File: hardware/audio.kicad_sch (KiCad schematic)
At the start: 3 parts, among them J5 AudioJack4

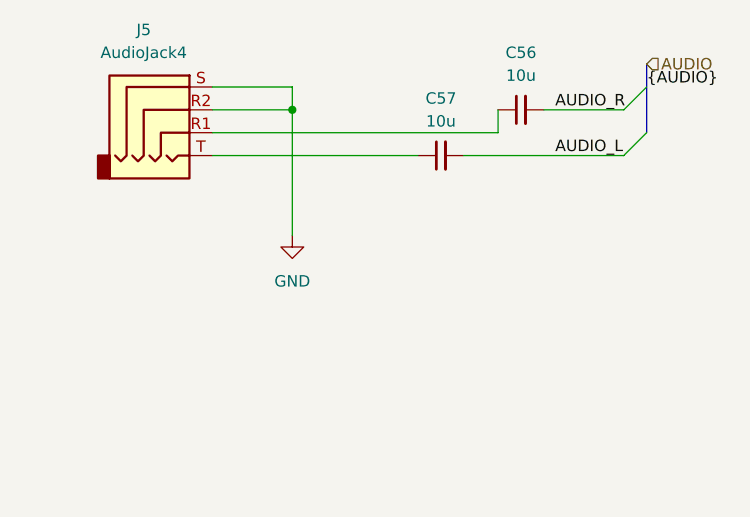
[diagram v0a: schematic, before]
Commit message: final touches
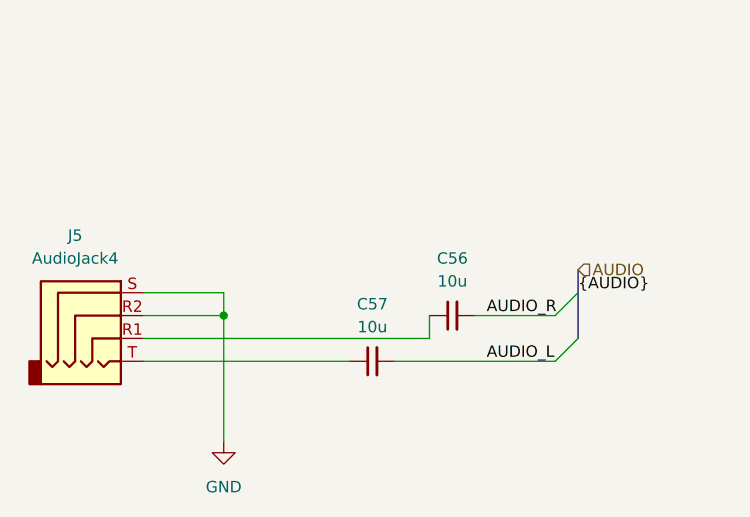
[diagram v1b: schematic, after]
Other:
- moved on the sheet: C56, C57, J5
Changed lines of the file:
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@@
 	(paper "A4")
 	(junction
-		(at 144.78 71.12)
+		(at 137.16 93.98)
 		(diameter 0)
 		(color 0 0 0 0)
 	)
 	(bus_entry
-		(at 184.15 73.66)
+		(at 176.53 96.52)
 		(size -2.54 2.54)
 		(stroke
@@
 	)
 	(bus_entry
-		(at 184.15 68.58)
+		(at 176.53 91.44)
 		(size -2.54 2.54)
 		(stroke
@@
 	(wire
 		(pts
-			(xy 135.89 71.12) (xy 144.78 71.12)
-		)
-		(stroke
-			(width 0)
-			(type default)
-		)
-	)
-	(wire
-		(pts
-			(xy 163.83 76.2) (xy 181.61 76.2)
-		)
-		(stroke
-			(width 0)
-			(type default)
-		)
-	)
-	(wire
-		(pts
-			(xy 144.78 85.09) (xy 144.78 71.12)
-		)
-		(stroke
-			(width 0)
-			(type default)
-		)
-	)
-	(wire
-		(pts
-			(xy 135.89 76.2) (xy 158.75 76.2)
+			(xy 128.27 93.98) (xy 137.16 93.98)
+		)
+		(stroke
+			(width 0)
+			(type default)
+		)
+	)
+	(wire
+		(pts
+			(xy 156.21 99.06) (xy 173.99 99.06)
+		)
+		(stroke
+			(width 0)
+			(type default)
+		)
+	)
+	(wire
+		(pts
+			(xy 137.16 107.95) (xy 137.16 93.98)
+		)
+		(stroke
+			(width 0)
+			(type default)
+		)
+	)
+	(wire
+		(pts
+			(xy 128.27 99.06) (xy 151.13 99.06)
 		)
 		(stroke
@@
 	(bus
 		(pts
-			(xy 184.15 66.04) (xy 184.15 73.66)
-		)
-		(stroke
-			(width 0)
-			(type default)
-		)
-	)
-	(wire
-		(pts
-			(xy 135.89 73.66) (xy 167.64 73.66)
-		)
-		(stroke
-			(width 0)
-			(type default)
-		)
-	)
-	(wire
-		(pts
-			(xy 135.89 68.58) (xy 144.78 68.58)
-		)
-		(stroke
-			(width 0)
-			(type default)
-		)
-	)
-	(wire
-		(pts
-			(xy 167.64 73.66) (xy 167.64 71.12)
-		)
-		(stroke
-			(width 0)
-			(type default)
-		)
-	)
-	(wire
-		(pts
-			(xy 172.72 71.12) (xy 181.61 71.12)
-		)
-		(stroke
-			(width 0)
-			(type default)
-		)
-	)
-	(wire
-		(pts
-			(xy 144.78 71.12) (xy 144.78 68.58)
+			(xy 176.53 88.9) (xy 176.53 96.52)
+		)
+		(stroke
+			(width 0)
+			(type default)
+		)
+	)
+	(wire
+		(pts
+			(xy 128.27 96.52) (xy 160.02 96.52)
+		)
+		(stroke
+			(width 0)
+			(type default)
+		)
+	)
+	(wire
+		(pts
+			(xy 128.27 91.44) (xy 137.16 91.44)
+		)
+		(stroke
+			(width 0)
+			(type default)
+		)
+	)
+	(wire
+		(pts
+			(xy 160.02 96.52) (xy 160.02 93.98)
+		)
+		(stroke
+			(width 0)
+			(type default)
+		)
+	)
+	(wire
+		(pts
+			(xy 165.1 93.98) (xy 173.99 93.98)
+		)
+		(stroke
+			(width 0)
+			(type default)
+		)
+	)
+	(wire
+		(pts
+			(xy 137.16 93.98) (xy 137.16 91.44)
 		)
 		(stroke
@@
 	)
 	(label "AUDIO_L"
-		(at 173.99 76.2 0)
+		(at 166.37 99.06 0)
 		(effects
 			(font
@@
 	)
 	(label "{AUDIO}"
-		(at 184.15 68.58 0)
+		(at 176.53 91.44 0)
 		(effects
 			(font
@@
 	)
 	(label "AUDIO_R"
-		(at 173.99 71.12 0)
+		(at 166.37 93.98 0)
 		(effects
 			(font
@@
 	(hierarchical_label "AUDIO"
 		(shape input)
-		(at 184.15 66.04 0)
+		(at 176.53 88.9 0)
 		(effects
 			(font
@@
 	(symbol
 		(lib_id "power:GND")
-		(at 144.78 85.09 0)
+		(at 137.16 107.95 0)
 		(unit 1)
 		(body_style 1)
@@
 		(fields_autoplaced yes)
 		(property "Reference" "#PWR055"
-			(at 144.78 91.44 0)
+			(at 137.16 114.3 0)
 			(hide yes)
 			(show_name no)
@@
 		)
 		(property "Value" "GND"
-			(at 144.78 90.17 0)
+			(at 137.16 113.03 0)
 			(show_name no)
 			(do_not_autoplace no)
@@
 		)
 		(property "Footprint" ""
-			(at 144.78 85.09 0)
+			(at 137.16 107.95 0)
 			(hide yes)
 			(show_name no)
@@
 		)
 		(property "Datasheet" ""
-			(at 144.78 85.09 0)
+			(at 137.16 107.95 0)
 			(hide yes)
 			(show_name no)
@@
 		)
 		(property "Description" "Power symbol creates a global label with name \"GND\" , ground"
-			(at 144.78 85.09 0)
+			(at 137.16 107.95 0)
 			(hide yes)
 			(show_name no)
@@
 	(symbol
 		(lib_id "Connector_Audio:AudioJack4")
-		(at 130.81 71.12 0)
+		(at 123.19 93.98 0)
 		(unit 1)
 		(body_style 1)
@@
 		(fields_autoplaced yes)
 		(property "Reference" "J5"
-			(at 128.27 62.23 0)
+			(at 120.65 85.09 0)
 			(show_name no)
 			(do_not_autoplace no)
@@
 		)
 		(property "Value" "AudioJack4"
-			(at 128.27 64.77 0)
+			(at 120.65 87.63 0)
 			(show_name no)
 			(do_not_autoplace no)
@@
 		)
 		(property "Footprint" "Connector_Audio:Jack_3.5mm_KoreanHropartsElec_PJ-320D-4A_Horizontal"
-			(at 130.81 71.12 0)
+			(at 123.19 93.98 0)
 			(hide yes)
 			(show_name no)
@@
 		)
 		(property "Datasheet" ""
-			(at 130.81 71.12 0)
+			(at 123.19 93.98 0)
 			(hide yes)
 			(show_name no)
@@
 		)
 		(property "Description" "Audio Jack, 4 Poles (TRRS)"
-			(at 130.81 71.12 0)
+			(at 123.19 93.98 0)
 			(hide yes)
 			(show_name no)
@@
 	(symbol
 		(lib_id "Device:C_Small")
-		(at 161.29 76.2 90)
+		(at 153.67 99.06 90)
 		(unit 1)
 		(body_style 1)
@@
 		(fields_autoplaced yes)
 		(property "Reference" "C57"
-			(at 161.2963 69.85 90)
+			(at 153.6763 92.71 90)
 			(show_name no)
 			(do_not_autoplace no)
@@
 		)
 		(property "Value" "10u"
-			(at 161.2963 72.39 90)
+			(at 153.6763 95.25 90)
 			(show_name no)
 			(do_not_autoplace no)
@@
 		)
 		(property "Footprint" "Capacitor_SMD:C_0603_1608Metric"
-			(at 161.29 76.2 0)
+			(at 153.67 99.06 0)
 			(hide yes)
 			(show_name no)
@@
 		)
 		(property "Datasheet" ""
-			(at 161.29 76.2 0)
+			(at 153.67 99.06 0)
 			(hide yes)
 			(show_name no)
@@
 		)
 		(property "Description" "Unpolarized capacitor, small symbol"
-			(at 161.29 76.2 0)
+			(at 153.67 99.06 0)
 			(hide yes)
 			(show_name no)
@@
 	(symbol
 		(lib_id "Device:C_Small")
-		(at 170.18 71.12 90)
+		(at 162.56 93.98 90)
 		(unit 1)
 		(body_style 1)
@@
 		(fields_autoplaced yes)
 		(property "Reference" "C56"
-			(at 170.1863 64.77 90)
+			(at 162.5663 87.63 90)
 			(show_name no)
 			(do_not_autoplace no)
@@
 		)
 		(property "Value" "10u"
-			(at 170.1863 67.31 90)
+			(at 162.5663 90.17 90)
 			(show_name no)
 			(do_not_autoplace no)
@@
 		)
 		(property "Footprint" "Capacitor_SMD:C_0603_1608Metric"
-			(at 170.18 71.12 0)
+			(at 162.56 93.98 0)
 			(hide yes)
 			(show_name no)
@@
 		)
 		(property "Datasheet" ""
-			(at 170.18 71.12 0)
+			(at 162.56 93.98 0)
 			(hide yes)
 			(show_name no)
@@
 		)
 		(property "Description" "Unpolarized capacitor, small symbol"
-			(at 170.18 71.12 0)
-			(hide yes)
-			(show_name no)
+			(at 162.56 93.98 0)
+			(hide yes)
+			(show_name no)
